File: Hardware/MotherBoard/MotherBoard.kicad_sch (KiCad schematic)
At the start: 25 parts, among them J1 POWER, J10 I/O_PWR, J13 USB_OTG, J2 I/O0, J5 I/O1, J6 EXTRN_CLCK, J9 Conn_02x02_Odd_Even, SW1 RESET_SW, SW2 ON_OFF, U1 AMS1117-5.0, X1 ACO-1MHz

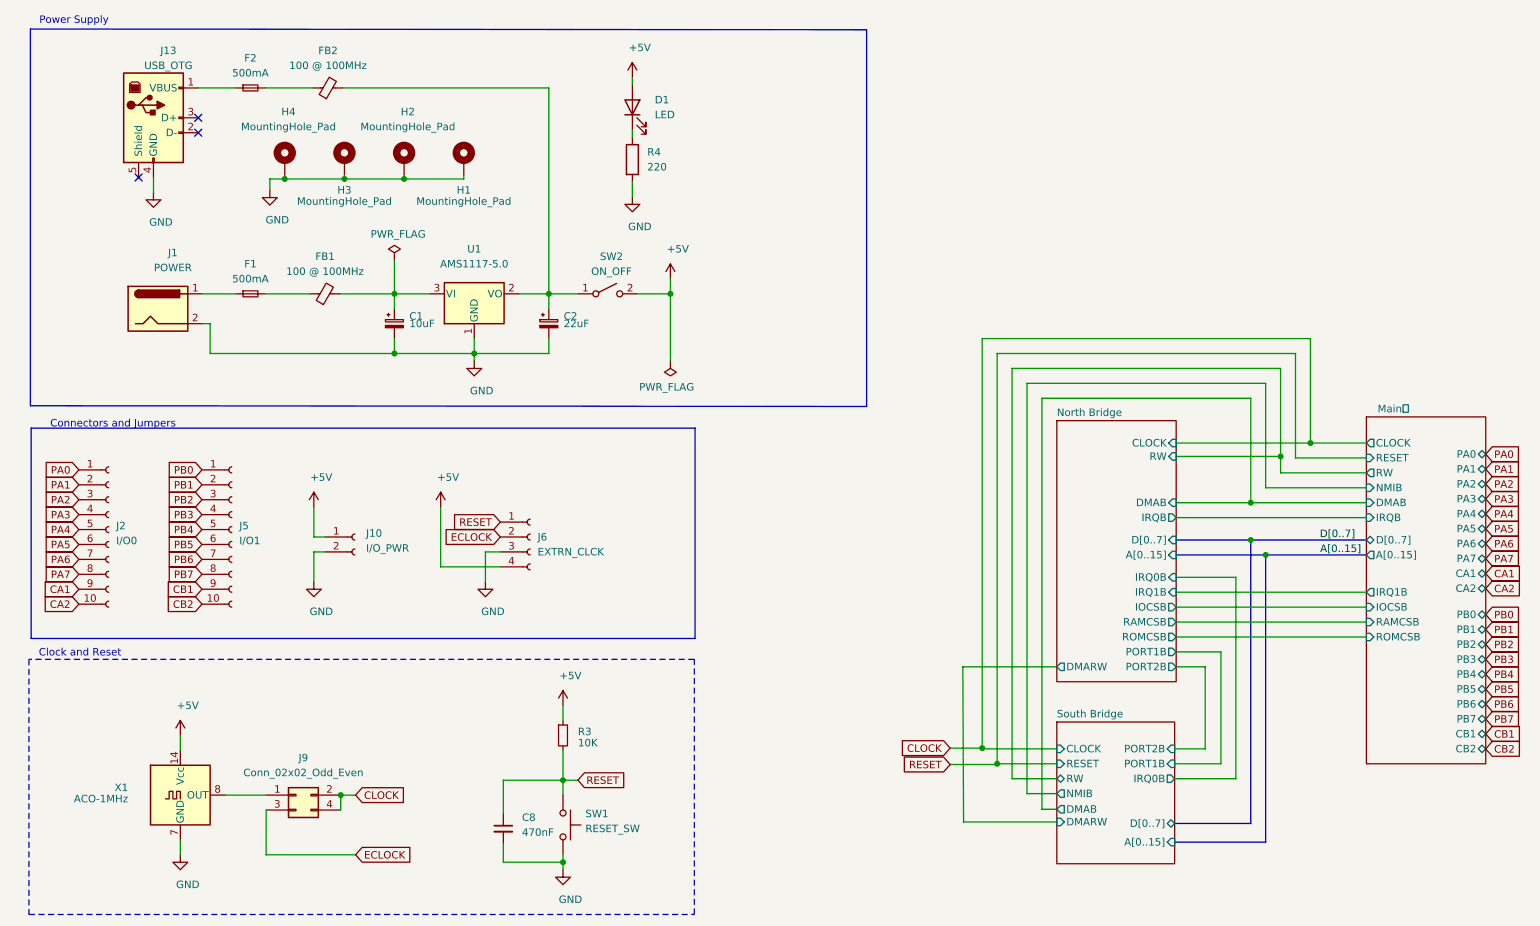
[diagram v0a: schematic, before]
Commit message: New motherboard version
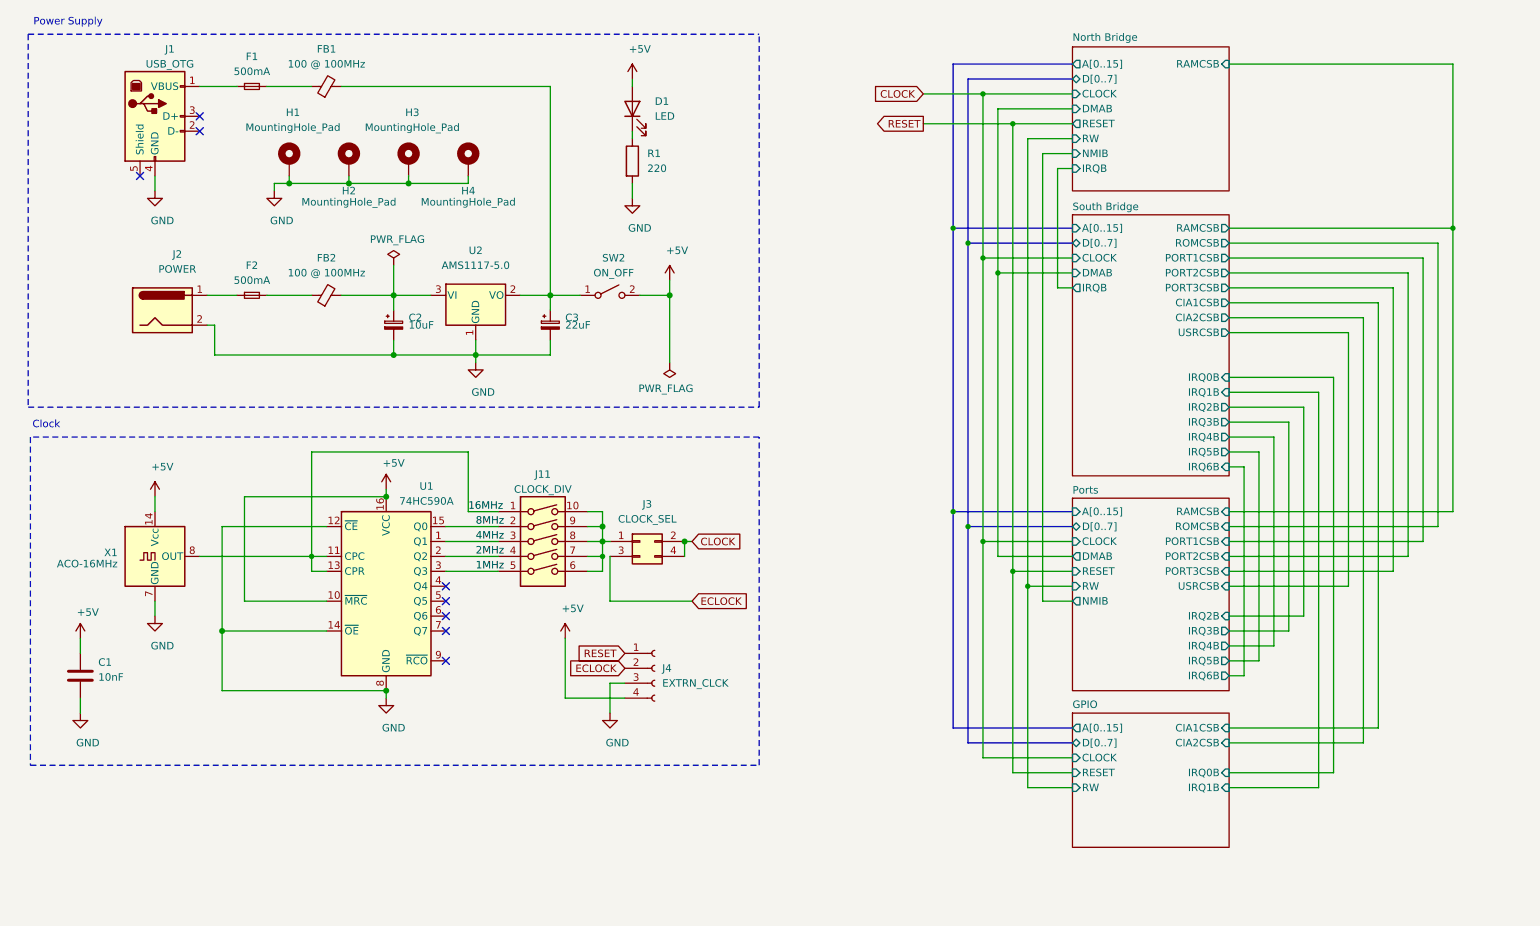
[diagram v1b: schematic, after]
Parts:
- removed C8: 470nF, Capacitor_THT:C_Disc_D5.0mm_W2.5mm_P5.00mm, symbol Device:C_Small
- removed J10: I/O_PWR, Connector_PinSocket_2.54mm:PinSocket_1x02_P2.54mm_Vertical, symbol Connector:Conn_01x02_Female
- removed J2: I/O0, Connector_PinSocket_2.54mm:PinSocket_1x10_P2.54mm_Vertical, symbol Connector:Conn_01x10_Female
- removed J5: I/O1, Connector_PinSocket_2.54mm:PinSocket_1x10_P2.54mm_Vertical, symbol Connector:Conn_01x10_Female
- removed R3: 10K, Resistor_THT:R_Axial_DIN0207_L6.3mm_D2.5mm_P10.16mm_Horizontal, symbol Device:R_Small
- removed SW1: RESET_SW, Button_Switch_THT:SW_Tactile_SPST_Angled_PTS645Vx83-2LFS, symbol Switch:SW_Push
- added C1: 10nF, Capacitor_THT:C_Disc_D5.0mm_W2.5mm_P2.50mm, symbol Device:C
- added J11: CLOCK_DIV, Button_Switch_THT:SW_DIP_SPSTx05_Slide_6.7x14.26mm_W7.62mm_P2.54mm_LowProfile, symbol Switch:SW_DIP_x05
- added U1: 74HC590A, Package_DIP:DIP-16_W7.62mm, symbol 74xx:74HC590A
- C2: renamed from C1; symbol Device:CP_Small -> Device:C_Polarized_Small
- C3: renamed from C2; symbol Device:CP_Small -> Device:C_Polarized_Small
- FB1: renamed from FB2; symbol Device:Ferrite_Bead_Small -> Device:FerriteBead_Small
- FB2: renamed from FB1; symbol Device:Ferrite_Bead_Small -> Device:FerriteBead_Small
- J3: renamed from J9; value Conn_02x02_Odd_Even -> CLOCK_SEL
- J4: renamed from J6; symbol Connector:Conn_01x04_Female -> Connector:Conn_01x04_Socket
- U2: renamed from U1; symbol Regulator_Linear:AMS1117-5.0 -> Regulator_Linear:AZ1117-5.0
- X1: value ACO-1MHz -> ACO-16MHz
- renumbered F2 to F1, F1 to F2, H4 to H1, H3 to H2, H2 to H3, H1 to H4, J13 to J1, J1 to J2, R4 to R1
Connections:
- net +5V: now also C1.1, U1.10 (~{MRC}), U1.16 (VCC)
- net GND: now also C1.2, U1.12 (~{CE}), U1.14 (~{OE}), U1.8 (GND)
- net at J3.1 (Pin_1): now also J11.10, J11.6, J11.7, J11.8, J11.9; no longer X1.8 (OUT)
- new net 16MHz: J11.1, U1.11 (CPC), U1.13 (CPR), X1.8 (OUT)
- new net 1MHz: J11.5, U1.3 (Q3)
- new net 2MHz: J11.4, U1.2 (Q2)
- new net 4MHz: J11.3, U1.1 (Q1)
- new net 8MHz: J11.2, U1.15 (Q0)
- no-connect marks 3 -> 8
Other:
- removed sheet Main 
- added sheet GPIO (gpio.kicad_sch)
- added sheet Ports (ports.kicad_sch)
- sheet North Bridge: file /home/romuald/Projects/Miniish/Hardware/MotherBoard/NorthBridge.kicad_sch -> NorthBridge.kicad_sch
- sheet North Bridge ports: added NMIB, RESET; removed DMARW, IOCSB, IRQ0B, IRQ1B, PORT1B, PORT2B, ROMCSB
- sheet South Bridge: file /home/romuald/Projects/Miniish/Hardware/MotherBoard/SouthBridge.kicad_sch -> SouthBridge.kicad_sch
- sheet South Bridge ports: added CIA1CSB, CIA2CSB, IRQ1B, IRQ2B, IRQ3B, IRQ4B, IRQ5B, IRQ6B, IRQB, PORT1CSB, PORT2CSB, PORT3CSB, RAMCSB, ROMCSB, USRCSB; removed DMARW, NMIB, PORT1B, PORT2B, RESET, RW
- note added: "Clock"
- note removed: "Clock and Reset"
- note removed: "Connectors and Jumpers"
- moved on the sheet: H1, H2, H3, H4, J2, J3, J4, X1
